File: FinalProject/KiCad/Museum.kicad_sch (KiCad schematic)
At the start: 10 parts, among them J1 Battery, M1 Stepper_Motor_bipolar, U1 ESP32C3, U2 ULN2003A, U3 SSD1306

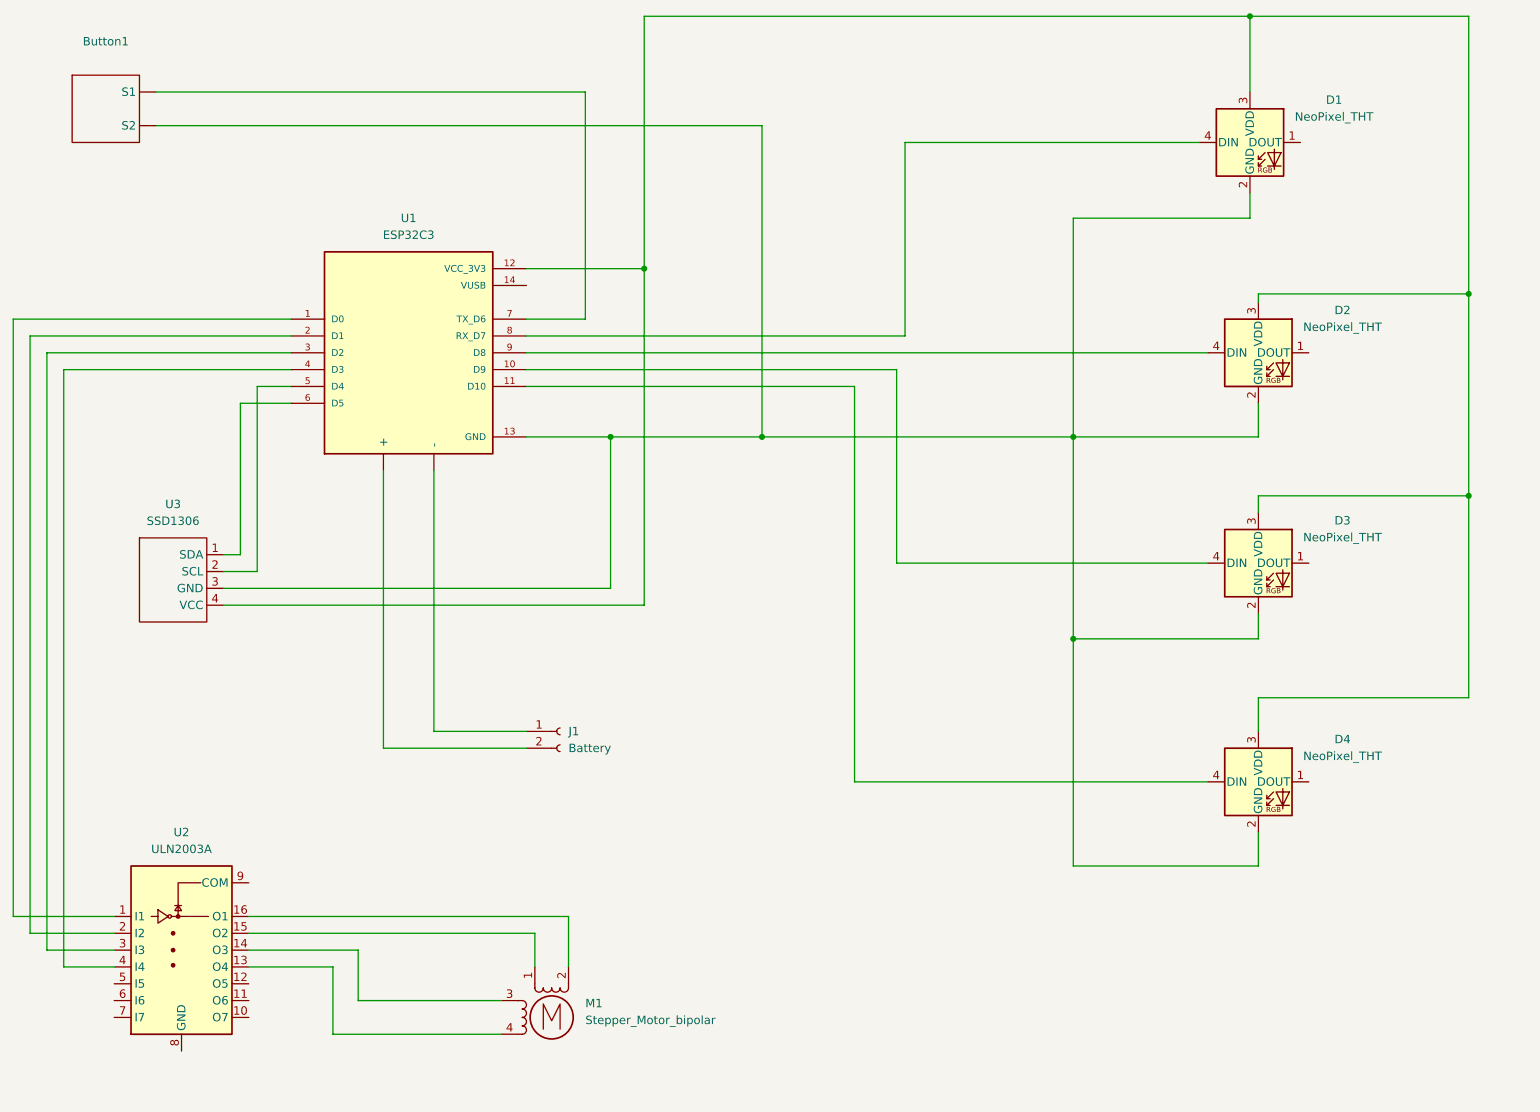
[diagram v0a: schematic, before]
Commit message: Lab5
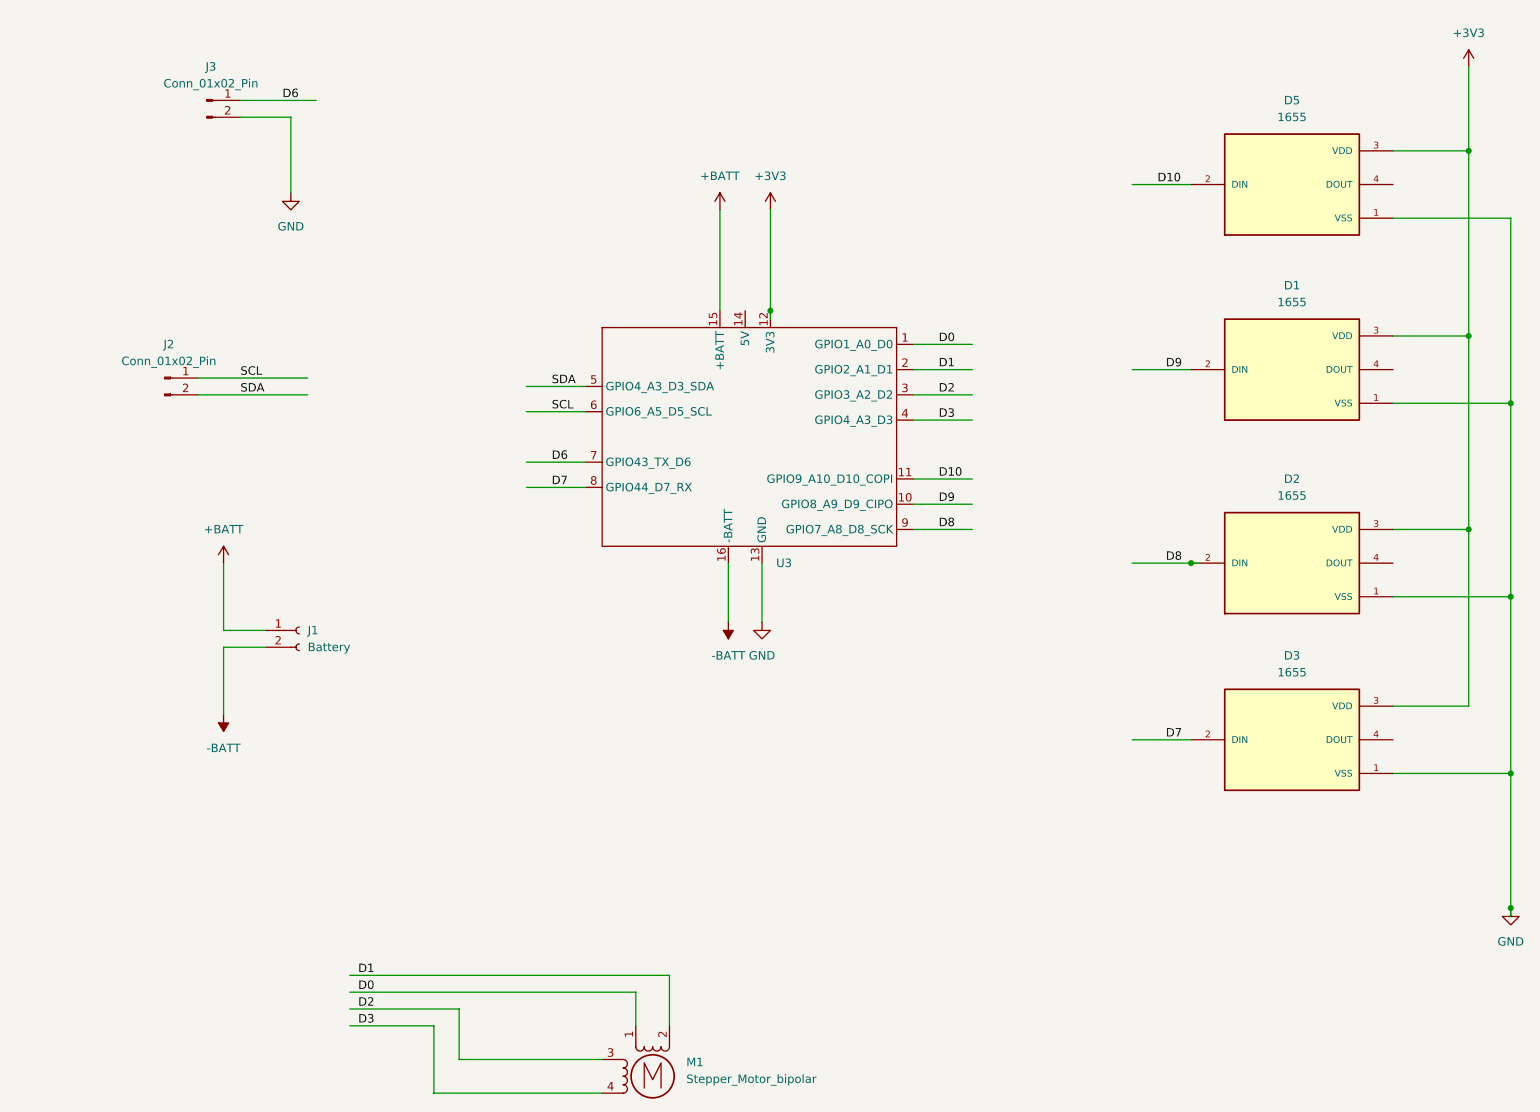
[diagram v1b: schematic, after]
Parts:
- removed Button1: ~, symbol Device:Button
- removed D1, D2, D3, D4: NeoPixel_THT, symbol LED:NeoPixel_THT
- removed U1: ESP32C3, 113991054:MODULE_113991054, symbol ESP32:113991054
- removed U2: ULN2003A, symbol Transistor_Array:ULN2003A
- removed U3: SSD1306, symbol Device:SDD1306
- added D1, D2, D3, D5: 1655, footprints:LED_1655, symbol LED1655:1655
- added J2, J3: Conn_01x02_Pin, Connector_PinHeader_1.00mm:PinHeader_1x02_P1.00mm_Vertical, symbol Connector:Conn_01x02_Pin
- added U3: ~, footprints:XIAO_ESP32, symbol GIX_ESP32:XIAO_ESP32
- J1: footprint (none) -> Connector_PinSocket_1.00mm:PinSocket_1x02_P1.00mm_Vertical
- M1: footprint (none) -> footprints:x27_stepper
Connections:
- net D3: now reaches M1.4
- net D3: now also U3.4 (GPIO4_A3_D3)
- net D2: now reaches M1.3
- net D2: now also U3.3 (GPIO3_A2_D2)
- net D0: now reaches M1.1
- net D0: now also U3.1 (GPIO1_A0_D0)
- net D1: now reaches M1.2 (-)
- net D1: now also U3.2 (GPIO2_A1_D1)
- net +BATT: now reaches J1.1 (Pin_1)
- net +BATT: now also U3.15 (+BATT)
- net -BATT: now reaches J1.2 (Pin_2)
- net -BATT: now also U3.16 (-BATT)
- new net +3V3: D1.3 (VDD), D2.3 (VDD), D3.3 (VDD), D5.3 (VDD), U3.12 (3V3)
- new net D10: D5.2 (DIN), U3.11 (GPIO9_A10_D10_COPI)
- new net D6: J3.1 (Pin_1), U3.7 (GPIO43_TX_D6)
- new net D7: D3.2 (DIN), U3.8 (GPIO44_D7_RX)
- new net D8: D2.2 (DIN), U3.9 (GPIO7_A8_D8_SCK)
- new net D9: D1.2 (DIN), U3.10 (GPIO8_A9_D9_CIPO)
- new net GND: D1.1 (VSS), D2.1 (VSS), D3.1 (VSS), D5.1 (VSS), J3.2 (Pin_2), U3.13 (GND)
- new net SCL: J2.1 (Pin_1), U3.6 (GPIO6_A5_D5_SCL)
- new net SDA: J2.2 (Pin_2), U3.5 (GPIO4_A3_D3_SDA)
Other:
- company: (none) -> Yuwen Chen
- title: (none) -> Museum Visitor Counter
- moved on the sheet: J1, M1
